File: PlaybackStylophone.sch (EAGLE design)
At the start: 51 parts, among them SW6 ON/OFF

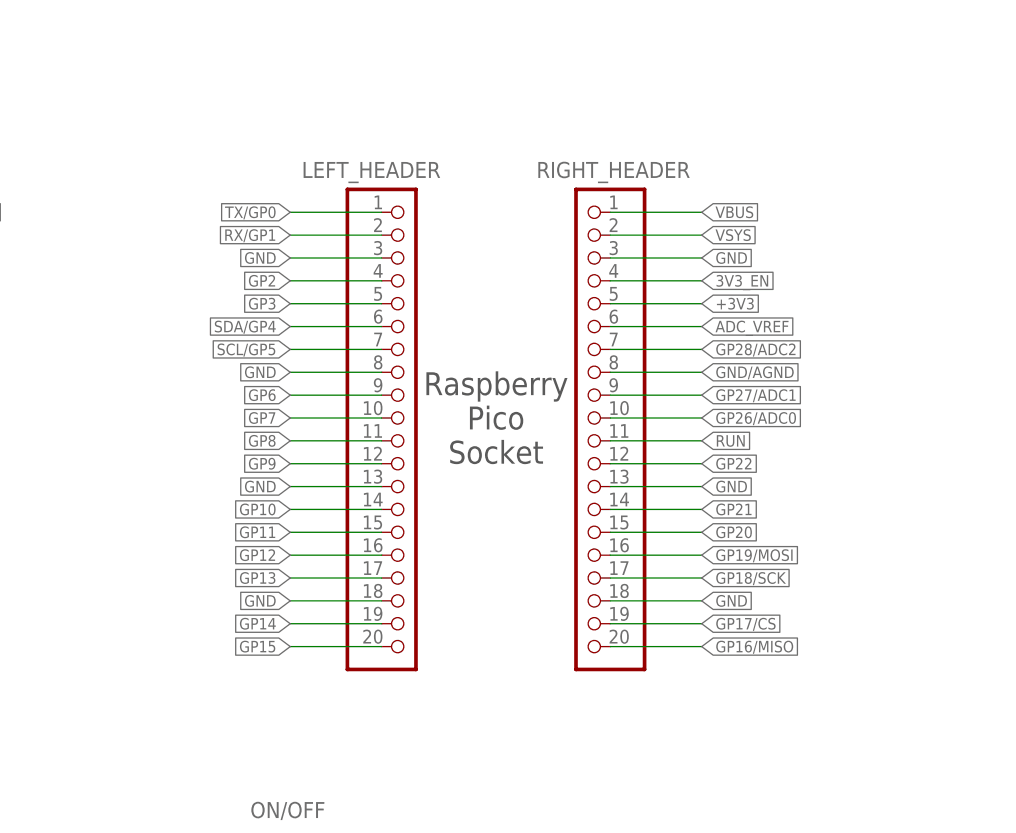
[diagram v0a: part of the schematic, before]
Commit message: Updated AUTODESK files
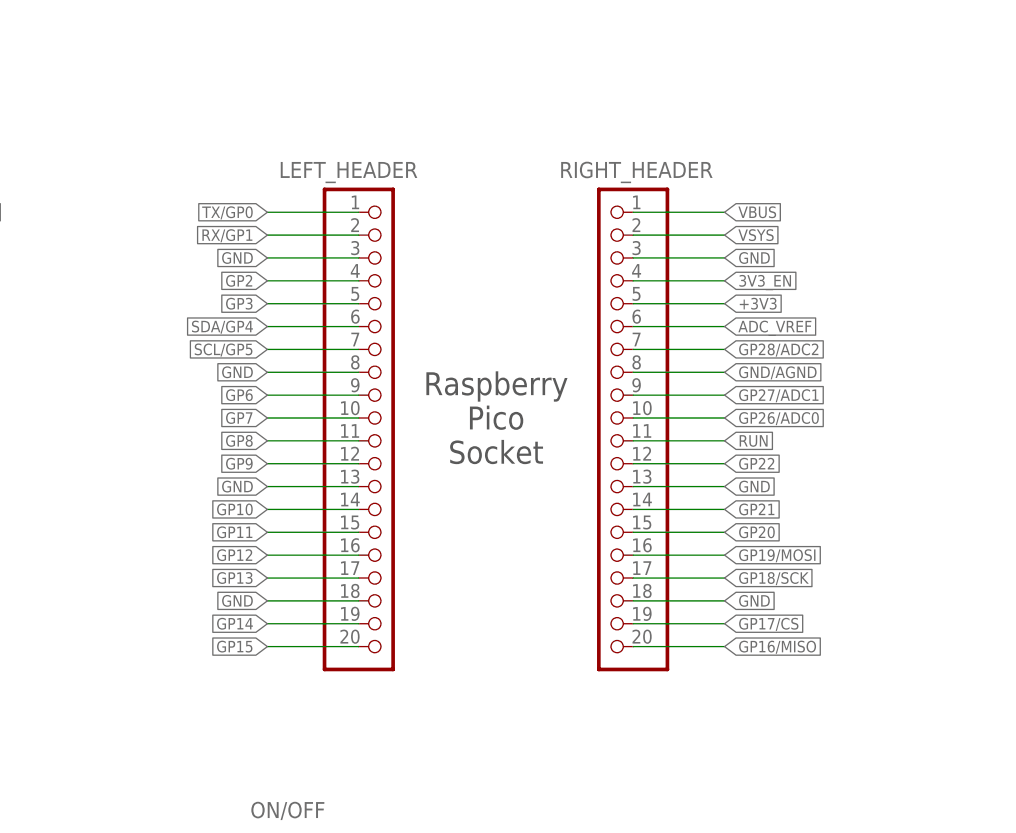
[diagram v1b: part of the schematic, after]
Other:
- moved on the sheet: LEFT_HEADER, RIGHT_HEADER
